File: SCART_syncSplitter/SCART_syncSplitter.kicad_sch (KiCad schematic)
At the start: 1 part, among them U1 EL1883

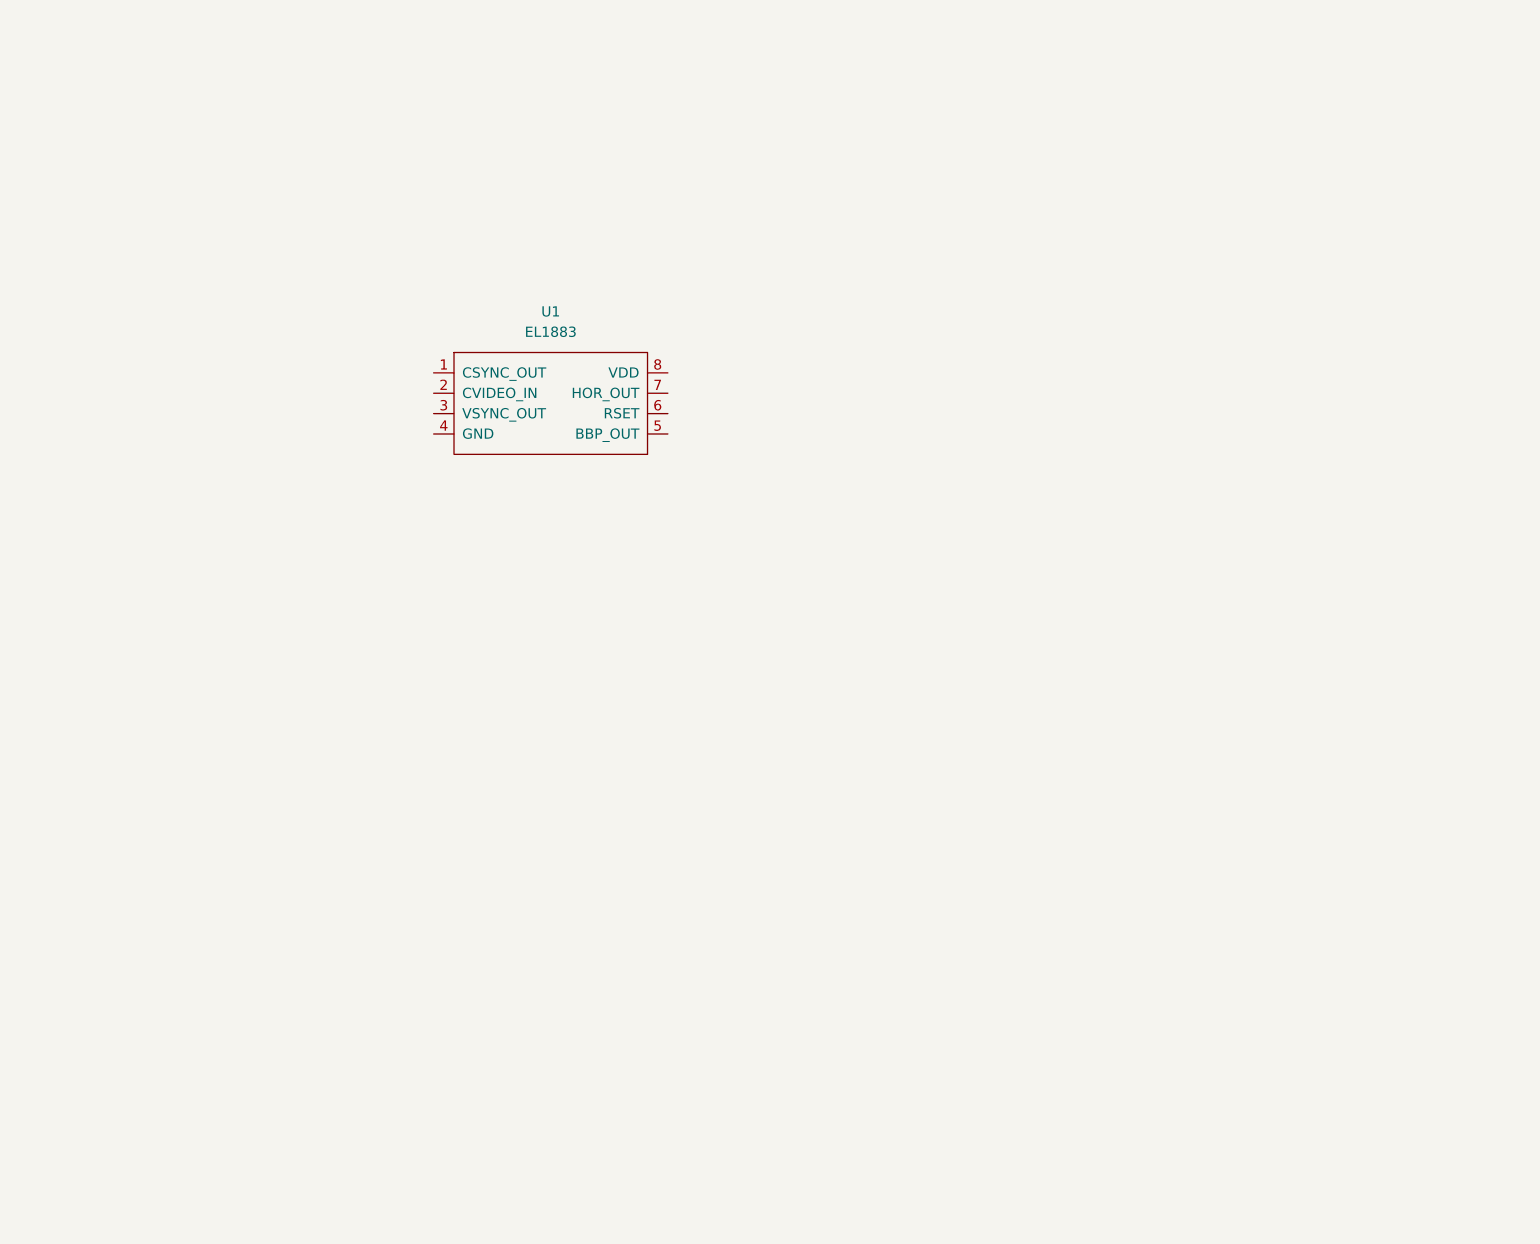
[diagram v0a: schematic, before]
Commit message: Update the schematic
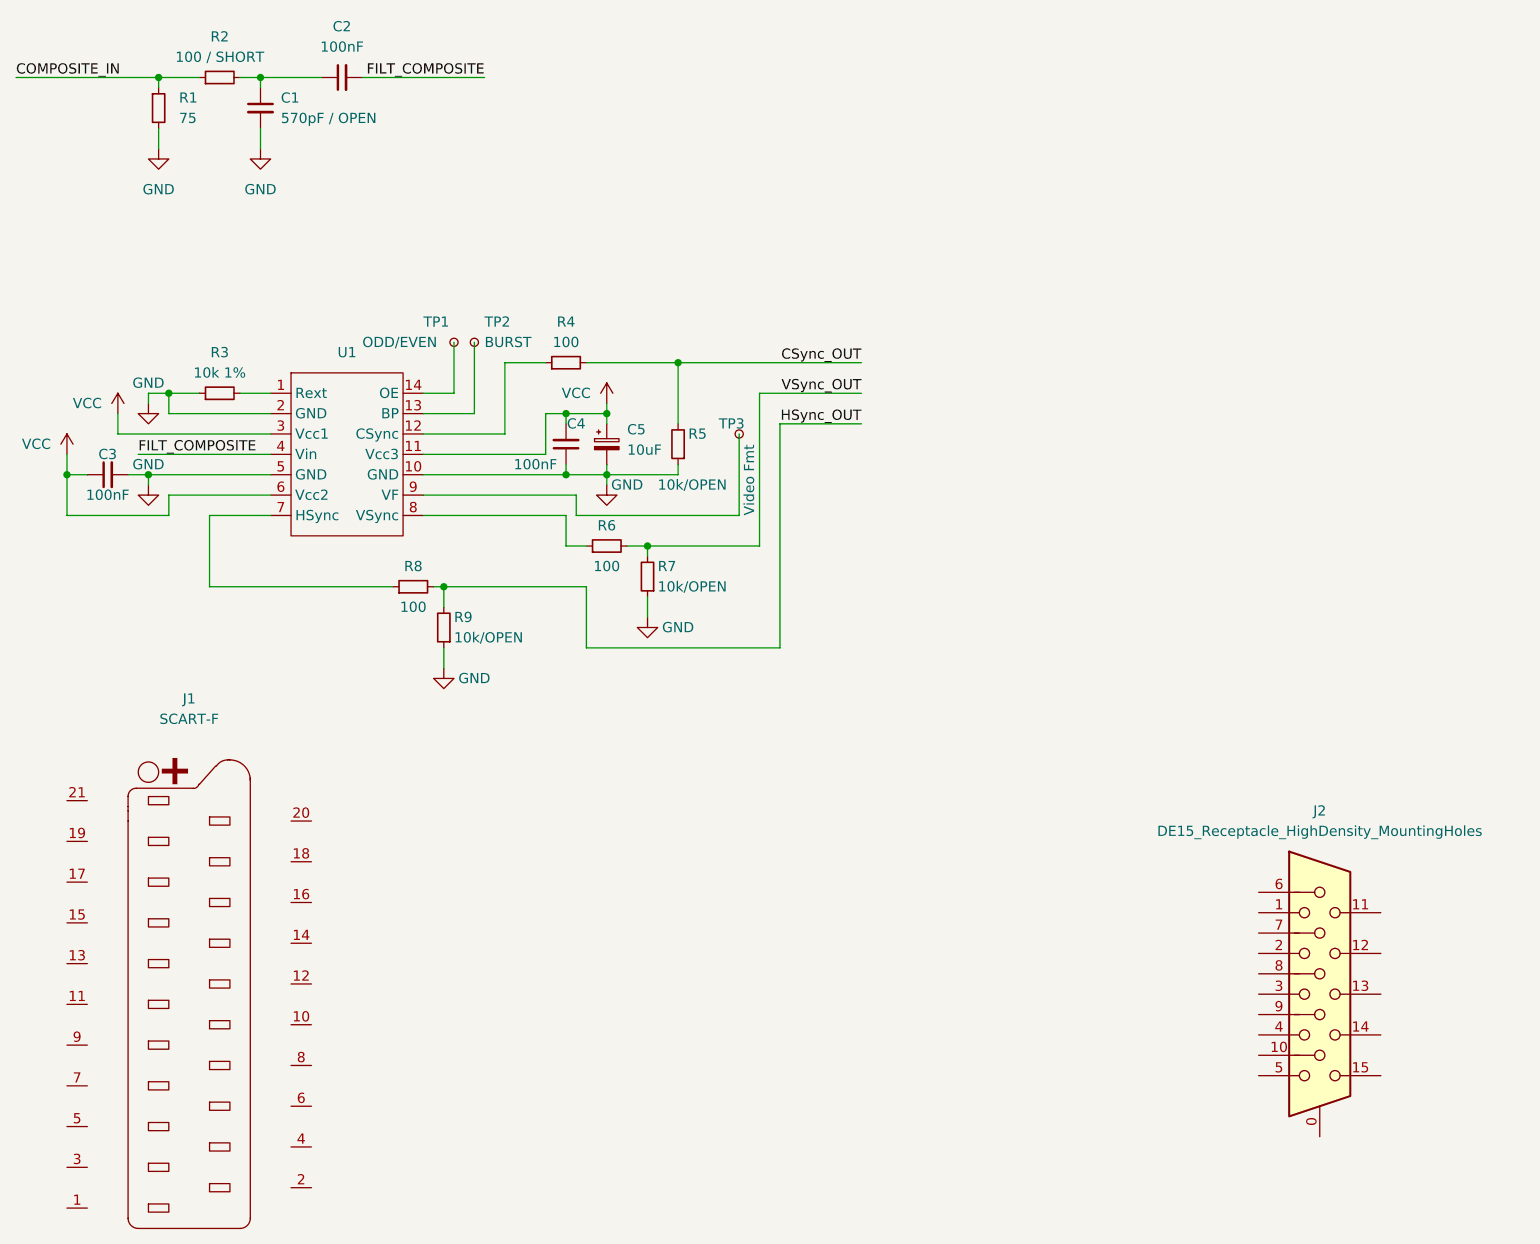
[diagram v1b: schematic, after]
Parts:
- removed U1: EL1883, Package_SO:SOP-8_3.9x4.9mm_P1.27mm, symbol EL1883:EL1883
- added C1: 570pF / OPEN, symbol Device:C_Small
- added C2, C3, C4: 100nF, symbol Device:C_Small
- added C5: 10uF, symbol Device:C_Polarized_Small
- added J1: SCART-F, symbol Connector:SCART-F
- added J2: DE15_Receptacle_HighDensity_MountingHoles, symbol Connector:DE15_Receptacle_HighDensity_MountingHoles
- added R1: 75, symbol Device:R_Small
- added R2: 100 / SHORT, symbol Device:R_Small
- added R3: 10k 1%, symbol Device:R_Small
- added R4, R6, R8: 100, symbol Device:R_Small
- added R5, R7, R9: 10k/OPEN, symbol Device:R_Small
- added TP1: ODD/EVEN, symbol Connector:TestPoint_Small
- added TP2: BURST, symbol Connector:TestPoint_Small
- added TP3: Video Fmt, symbol Connector:TestPoint_Small
- added U1: ~, Package_SO:TSSOP-14_4.4x5mm_P0.65mm, symbol LMH1981:LMH1981
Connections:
- new net: TP1.1, U1.14 (OE)
- new net: R3.2, U1.1 (Rext)
- new net: C1.1, C2.1, R2.2
- new net: R8.1, U1.7 (HSync)
- new net: R4.1, U1.12 (CSync)
- new net: TP2.1, U1.13 (BP)
- new net: R6.1, U1.8 (VSync)
- new net: TP3.1, U1.9 (VF)
- new net COMPOSITE_IN: R1.1, R2.1
- new net CSync_OUT: R4.2, R5.2
- new net FILT_COMPOSITE: C2.2, U1.4 (Vin)
- new net GND: C1.2, C3.2, C4.1, C5.2, R1.2, R3.1, R5.1, R7.1, R9.1, U1.10 (GND), U1.2 (GND), U1.5 (GND)
- new net HSync_OUT: R8.2, R9.2
- new net VCC: C3.1, C4.2, C5.1, U1.11 (Vcc3), U1.3 (Vcc1), U1.6 (Vcc2)
- new net VSync_OUT: R6.2, R7.2
